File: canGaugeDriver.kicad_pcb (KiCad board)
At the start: 2 copper layers, 80 x 41.4 mm, 46 parts, among them J1 CANbed 1.0 Interface, J3 348260240, J4 DB9'MEAL', U1 TPL7407LA, U2 TPL7407LA

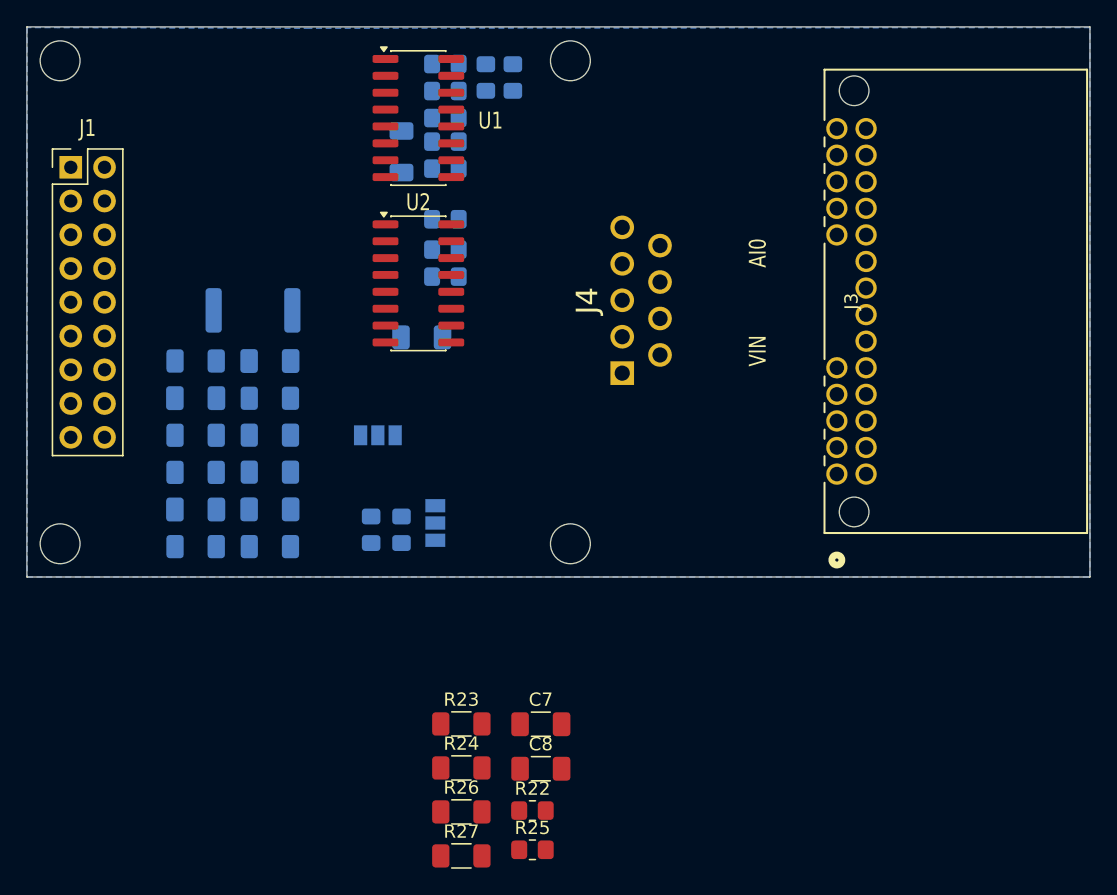
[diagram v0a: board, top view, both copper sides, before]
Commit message: routed board
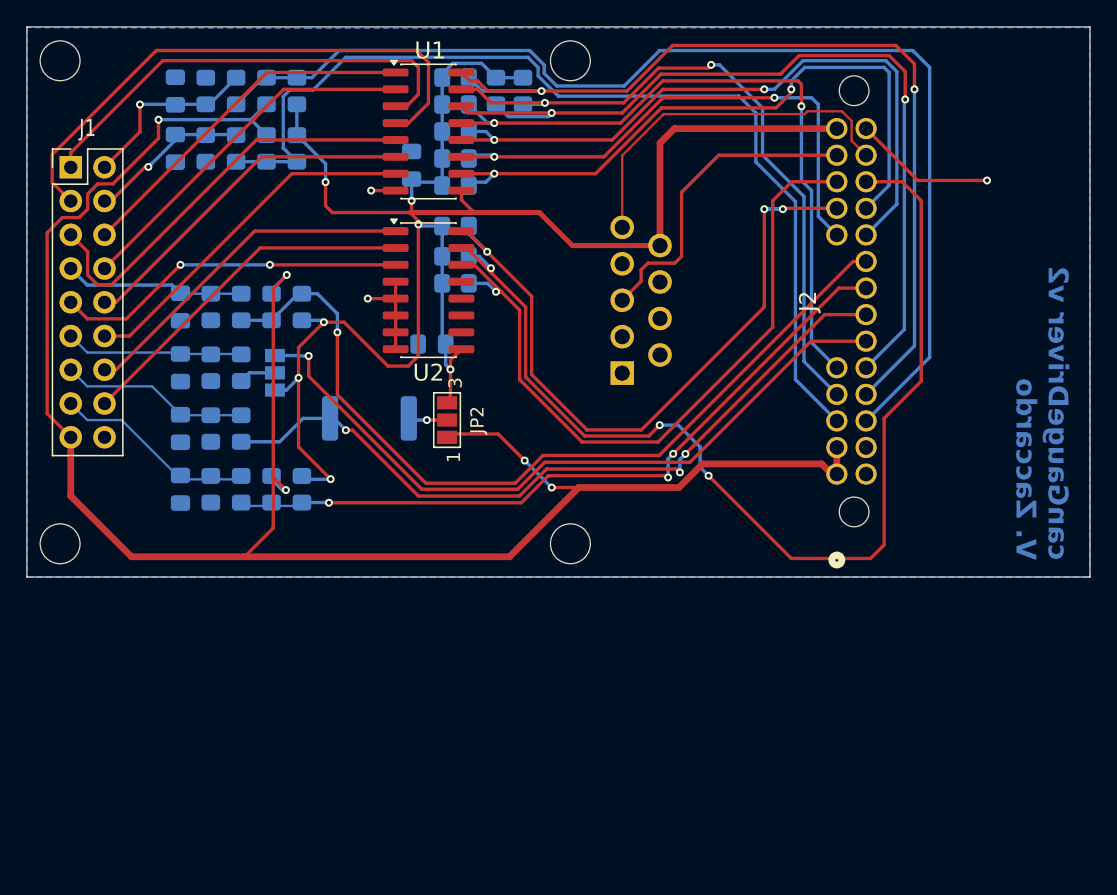
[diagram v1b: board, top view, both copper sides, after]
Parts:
- added R10: 10k, Resistor_SMD:R_0805_2012Metric_Pad1.20x1.40mm_HandSolder, B.Cu at (120.0, 95.1)
- added R11: 10k, Resistor_SMD:R_0805_2012Metric_Pad1.20x1.40mm_HandSolder, B.Cu at (120.0, 81.4)
- added R14: 10k, Resistor_SMD:R_0805_2012Metric_Pad1.20x1.40mm_HandSolder, B.Cu at (121.9, 69.5)
- added R2: 10k, Resistor_SMD:R_0805_2012Metric_Pad1.20x1.40mm_HandSolder, B.Cu at (121.9, 65.2)
- C1, C2: footprint Capacitor_SMD:C_1206_3216Metric_Pad1.33x1.80mm_HandSolder -> Capacitor_SMD:C_0805_2012Metric_Pad1.18x1.45mm_HandSolder
- C3: renamed from C7; footprint Capacitor_SMD:C_1206_3216Metric_Pad1.33x1.80mm_HandSolder -> Capacitor_SMD:C_0805_2012Metric_Pad1.18x1.45mm_HandSolder; moved to B.Cu
- C4: renamed from C3; footprint Capacitor_SMD:C_1206_3216Metric_Pad1.33x1.80mm_HandSolder -> Capacitor_SMD:C_0805_2012Metric_Pad1.18x1.45mm_HandSolder
- C5: renamed from C4; footprint Capacitor_SMD:C_1206_3216Metric_Pad1.33x1.80mm_HandSolder -> Capacitor_SMD:C_0805_2012Metric_Pad1.18x1.45mm_HandSolder
- C6: renamed from C8; footprint Capacitor_SMD:C_1206_3216Metric_Pad1.33x1.80mm_HandSolder -> Capacitor_SMD:C_0805_2012Metric_Pad1.18x1.45mm_HandSolder; moved to B.Cu
- C7: renamed from C6; footprint Capacitor_SMD:C_1206_3216Metric_Pad1.33x1.80mm_HandSolder -> Capacitor_SMD:C_0805_2012Metric_Pad1.18x1.45mm_HandSolder
- C8: renamed from C5; footprint Capacitor_SMD:C_1206_3216Metric_Pad1.33x1.80mm_HandSolder -> Capacitor_SMD:C_0805_2012Metric_Pad1.18x1.45mm_HandSolder
- JP2: moved to F.Cu
- R15: renamed from R25; moved to B.Cu
- R16: renamed from R5; footprint Resistor_SMD:R_1206_3216Metric_Pad1.30x1.75mm_HandSolder -> Resistor_SMD:R_0805_2012Metric_Pad1.20x1.40mm_HandSolder
- R17: renamed from R6; footprint Resistor_SMD:R_1206_3216Metric_Pad1.30x1.75mm_HandSolder -> Resistor_SMD:R_0805_2012Metric_Pad1.20x1.40mm_HandSolder
- R18: renamed from R7; footprint Resistor_SMD:R_1206_3216Metric_Pad1.30x1.75mm_HandSolder -> Resistor_SMD:R_0805_2012Metric_Pad1.20x1.40mm_HandSolder
- R19: renamed from R8; footprint Resistor_SMD:R_1206_3216Metric_Pad1.30x1.75mm_HandSolder -> Resistor_SMD:R_0805_2012Metric_Pad1.20x1.40mm_HandSolder
- R20: renamed from R26; footprint Resistor_SMD:R_1206_3216Metric_Pad1.30x1.75mm_HandSolder -> Resistor_SMD:R_0805_2012Metric_Pad1.20x1.40mm_HandSolder; moved to B.Cu
- R21: renamed from R27; footprint Resistor_SMD:R_1206_3216Metric_Pad1.30x1.75mm_HandSolder -> Resistor_SMD:R_0805_2012Metric_Pad1.20x1.40mm_HandSolder; moved to B.Cu
- R3: renamed from R22; moved to B.Cu
- R4: renamed from R1; footprint Resistor_SMD:R_1206_3216Metric_Pad1.30x1.75mm_HandSolder -> Resistor_SMD:R_0805_2012Metric_Pad1.20x1.40mm_HandSolder
- R5: renamed from R2; footprint Resistor_SMD:R_1206_3216Metric_Pad1.30x1.75mm_HandSolder -> Resistor_SMD:R_0805_2012Metric_Pad1.20x1.40mm_HandSolder
- R6: renamed from R3; footprint Resistor_SMD:R_1206_3216Metric_Pad1.30x1.75mm_HandSolder -> Resistor_SMD:R_0805_2012Metric_Pad1.20x1.40mm_HandSolder
- R7: renamed from R4; footprint Resistor_SMD:R_1206_3216Metric_Pad1.30x1.75mm_HandSolder -> Resistor_SMD:R_0805_2012Metric_Pad1.20x1.40mm_HandSolder
- R8: renamed from R23; value 30.1k -> 0; footprint Resistor_SMD:R_1206_3216Metric_Pad1.30x1.75mm_HandSolder -> Resistor_SMD:R_0805_2012Metric_Pad1.20x1.40mm_HandSolder; moved to B.Cu
- R9: renamed from R24; value 9.76k -> DNP; footprint Resistor_SMD:R_1206_3216Metric_Pad1.30x1.75mm_HandSolder -> Resistor_SMD:R_0805_2012Metric_Pad1.20x1.40mm_HandSolder; moved to B.Cu
- moved R3 57.7 mm to (119.6, 65.2), turned to -90 degrees
- moved R21 56.6 mm to (115.1, 69.5), turned to -90 degrees
- moved R15 56.5 mm to (119.6, 69.5), turned to 90 degrees
- moved C3 55.0 mm to (112.8, 65.2), turned to 90 degrees
- moved R9 54.5 mm to (115.1, 65.2), turned to 90 degrees
- moved C6 54.2 mm to (112.8, 69.5), turned to -90 degrees
- moved R20 52.7 mm to (117.3, 69.5), turned to 90 degrees
- moved R8 50.6 mm to (117.3, 65.2), turned to 90 degrees
- moved R12 18.4 mm to (122.3, 81.4), turned to -90 degrees
- moved R18 18.4 mm to (117.7, 81.4), turned to 90 degrees
- moved C5 15.3 mm to (113.2, 81.4), turned to -90 degrees
- moved R19 12.5 mm to (115.4, 81.4), turned to -90 degrees
- moved R1 12.0 mm to (127.4, 89.8)
- moved JP1 9.06 mm to (120.3, 86.4), turned to -90 degrees
- moved JP2 7.80 mm to (133.2, 89.9)
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- renumbered J4 to DB1, J3 to J2, R19 to R1, R20 to R12, R21 to R13, R10 to R22, R9 to R23, R11 to R24, R12 to R25, R14 to R26, R15 to R27, R13 to R28, R16 to R29, R17 to R30, R18 to R31
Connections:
- J2 pad 13: /D2_OUT -> /D0_IN
- J2 pad 14: /D4_OUT -> /D2_OUT
- J2 pad 15: /D6_OUT -> /D4_OUT
- J2 pad 20: /D9_OUT -> /D6_OUT
- J2 pad 21: /D11_OUT -> /D9_OUT
- J2 pad 22: GND -> /D11_OUT
- J2 pad 3: /D3_OUT -> /D1_IN
- J2 pad 4: /D5_OUT -> /D3_OUT
- J2 pad 5: /D8_OUT -> /D5_OUT
- J2 pad 6: /D10_OUT -> /D8_OUT
- J2 pad 7: /D12_OUT -> /D10_OUT
- J2 pad 8: /5V -> /D12_OUT
- R1 pad 2: /5V -> Net-(JP2-C)
- R12 pad 2: Net-(JP2-C) -> /VIN
- R15 pad 1: /AI2 -> /D1_IN
- R15 pad 2: /VIN -> /5V
- R20 pad 1: /AI2 -> /D1_IN
- R22 pad 1: /VIN -> /D2_OUT
- R22 pad 2: /D2_OUT -> /VIN
- R3 pad 1: /AI2 -> /D0_IN
- R3 pad 2: /VIN -> /5V
- R8 pad 1: /AI2 -> /D0_IN
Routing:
- net /5V: track 0.00 -> 147.8 mm, vias 0 -> 5
- net /VIN: track 0.00 -> 133.8 mm, vias 0 -> 7
- net /D0_IN: track 0.00 -> 85.6 mm
- net /D11_OUT: track 0.00 -> 80.5 mm, vias 0 -> 3
- net /D1_IN: track 0.00 -> 74.5 mm
- net /D2_OUT: track 0.00 -> 68.9 mm, vias 0 -> 2
- net /D4_OUT: track 0.00 -> 64.1 mm, vias 0 -> 2
- net /AI3: track 0.00 -> 64.0 mm, vias 0 -> 1
- net /AI1: track 0.00 -> 56.1 mm, vias 0 -> 3
- net /AI2: track 0.00 -> 54.9 mm, vias 0 -> 3
- net /AI0: track 0.00 -> 54.2 mm, vias 0 -> 1
- net /D12_OUT: track 0.00 -> 53.2 mm, vias 0 -> 1
- net /D5_OUT: track 0.00 -> 51.9 mm, vias 0 -> 2
- net /D10_OUT: track 0.00 -> 51.6 mm, vias 0 -> 3
- net /D3_OUT: track 0.00 -> 51.2 mm, vias 0 -> 2
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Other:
- board text added: "canGaugeDriver v2 V. Zaccardo"
- board text removed: "AI0"
- board text removed: "VIN"
